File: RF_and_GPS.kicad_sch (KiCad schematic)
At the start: 34 parts, among them J12 U.FL-R-SMT-1, J2 U.FL-R-SMT-1, J29 Conn_02x05_Odd_Even, J7 U.FL-R-SMT-1, Q21 IRF7404, Q38 IRLML2803, Q9 IRLML2803, SW2 KMR231NG LFS, U11 MAX706RESA+, U13 EP2W+, U14 S1216V8, U23 RFM98PW, U9 ATSAMD21E18A-A

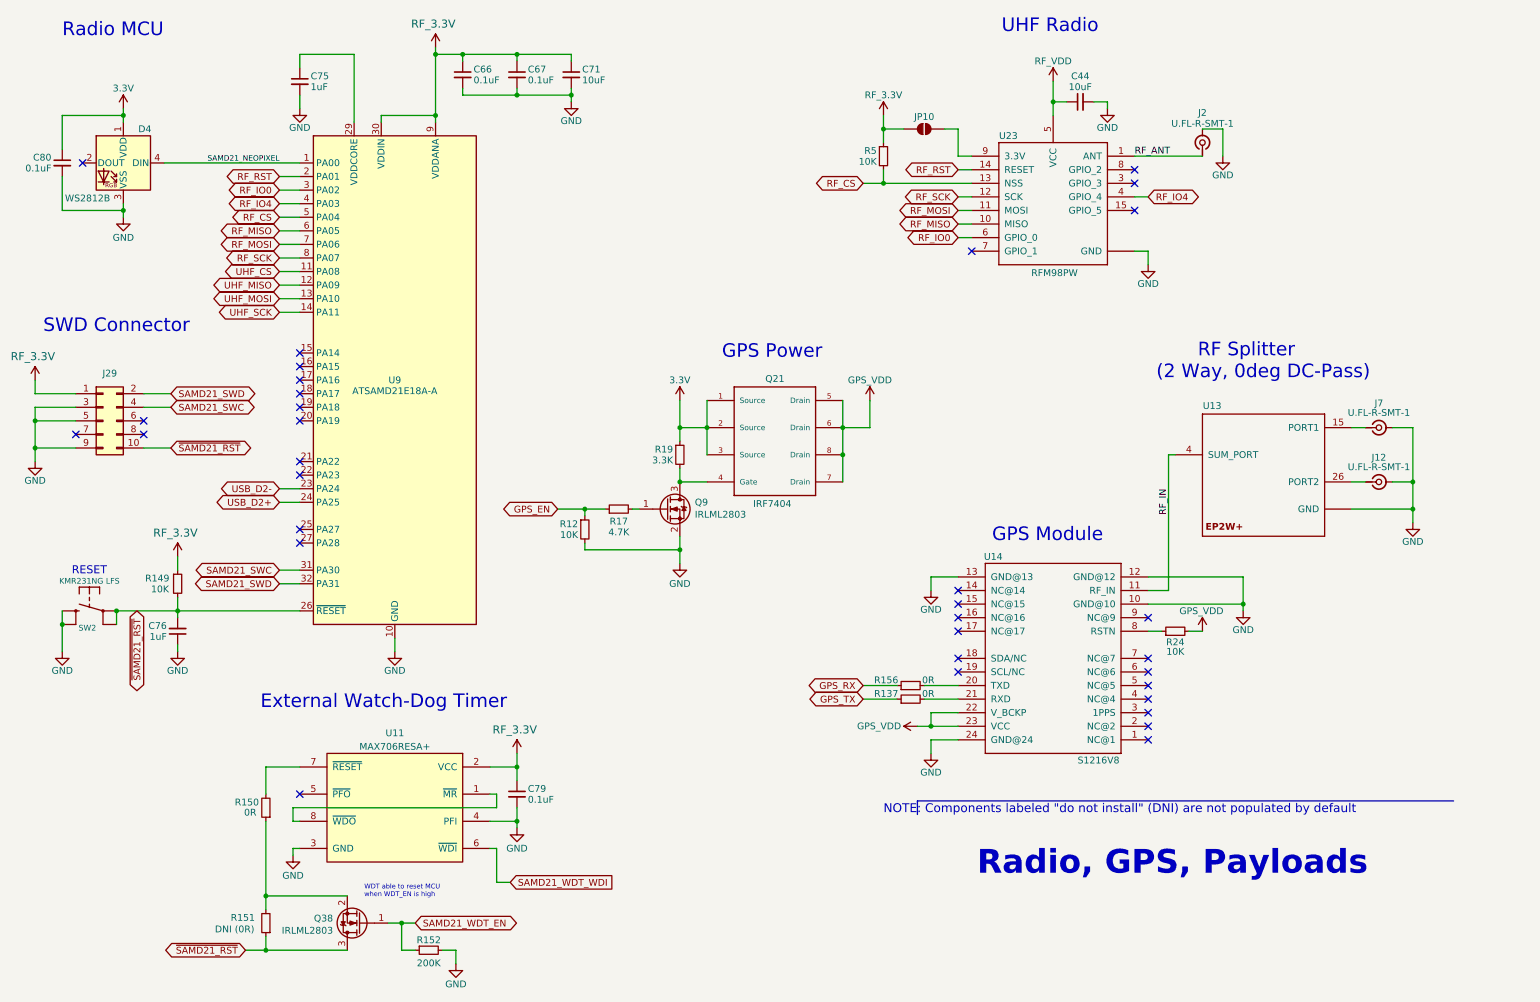
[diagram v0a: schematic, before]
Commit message: Complete layout
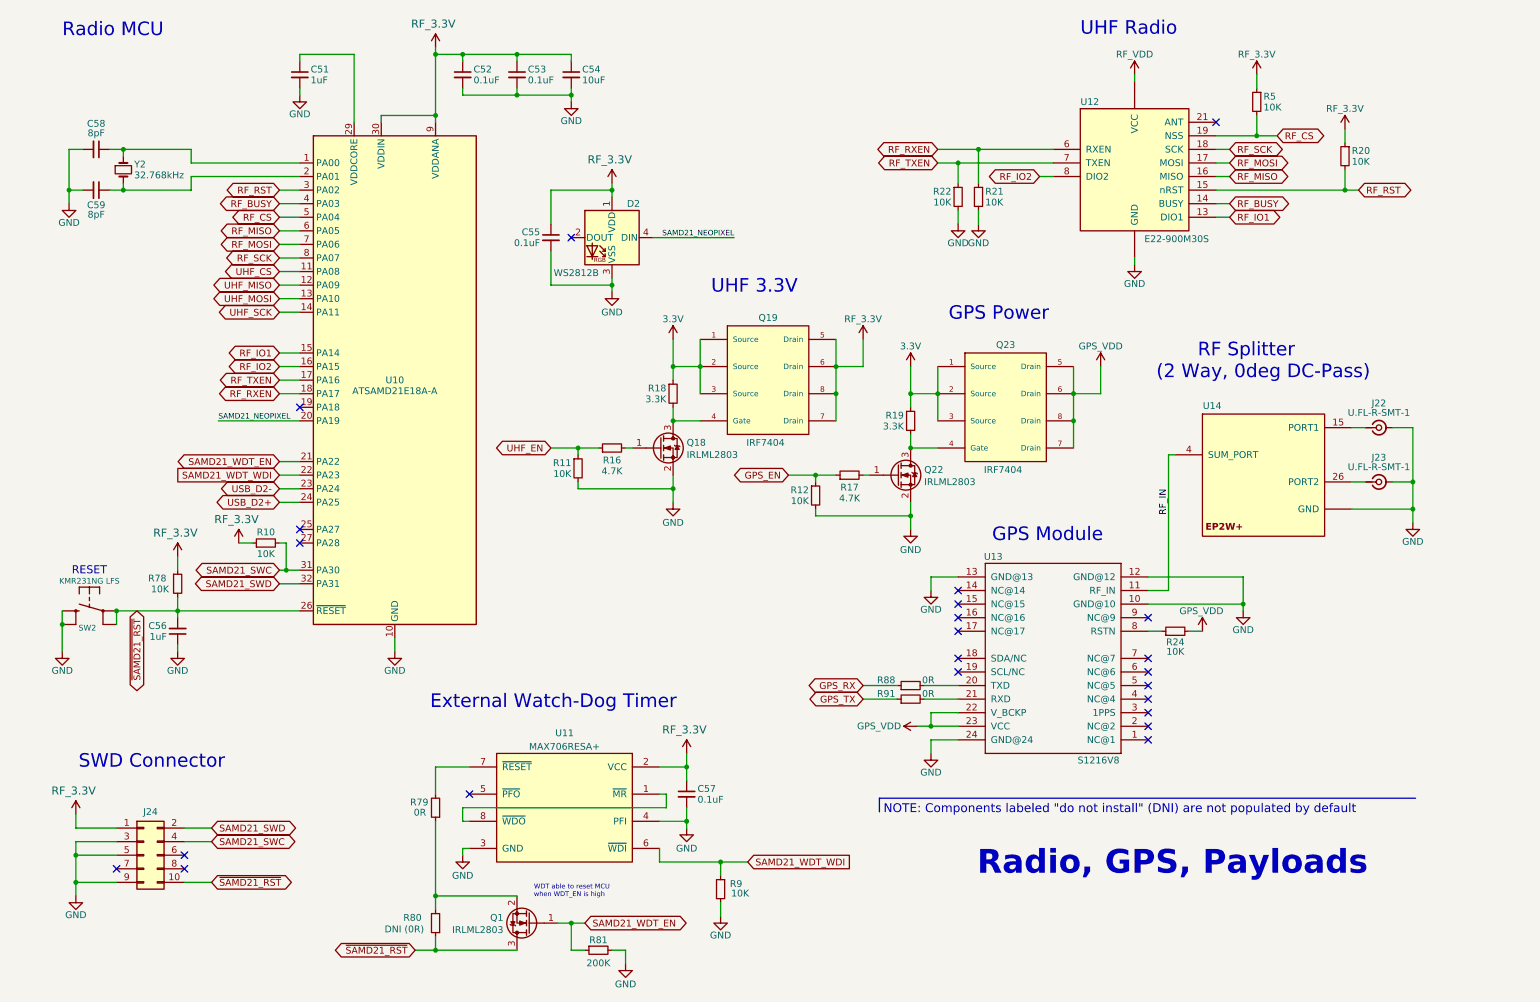
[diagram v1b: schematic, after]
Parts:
- removed C44: 10uF, symbol Device:C_Small
- removed J2: U.FL-R-SMT-1, symbol Connector:Conn_Coaxial_Small
- removed JP10: SolderJumper_2_Open, symbol Jumper:SolderJumper_2_Open
- added C58, C59: 8pF, Capacitor_SMD:C_0603_1608Metric, symbol Device:C_Small
- added Q18: IRLML2803, Package_TO_SOT_SMD:SOT-23, symbol Mainboard:IRLML2803
- added Q19: IRF7404, Package_SO:SOIC-8_3.9x4.9mm_P1.27mm, symbol Mainboard:IRF7404
- added R10, R11, R20, R21, R22, R9: 10K, Resistor_SMD:R_0603_1608Metric, symbol Device:R_Small
- added R16: 4.7K, Resistor_SMD:R_0603_1608Metric, symbol Device:R_Small
- added R18: 3.3K, Resistor_SMD:R_0603_1608Metric, symbol Device:R_Small
- added Y2: 32.768kHz, Crystal:Crystal_SMD_3215-2Pin_3.2x1.5mm, symbol Device:Crystal_Small
- C51: renamed from C75; footprint (none) -> Capacitor_SMD:C_0603_1608Metric
- C52: renamed from C66; footprint (none) -> Capacitor_SMD:C_0603_1608Metric
- C53: renamed from C67; footprint (none) -> Capacitor_SMD:C_0603_1608Metric
- C54: renamed from C71; footprint (none) -> Capacitor_SMD:C_0603_1608Metric
- C55: renamed from C80; symbol mainboard:C_Small -> Device:C_Small
- C56: renamed from C76; symbol mainboard:C_Small -> Device:C_Small
- J22: renamed from J7; footprint (none) -> Connector_Coaxial:U.FL_Hirose_U.FL-R-SMT-1_Vertical
- J23: renamed from J12; footprint (none) -> Connector_Coaxial:U.FL_Hirose_U.FL-R-SMT-1_Vertical
- J24: renamed from J29; footprint (none) -> Connector_PinHeader_1.27mm:PinHeader_2x05_P1.27mm_Vertical_SMD
- Q1: renamed from Q38; symbol Transistor_FET:IRLML2060 -> Mainboard:IRLML2803
- Q22: renamed from Q9; symbol Transistor_FET:IRLML2060 -> Mainboard:IRLML2803
- Q23: renamed from Q21; footprint mainboard:NDS8434 -> Package_SO:SOIC-8_3.9x4.9mm_P1.27mm; symbol mainboard:NDS8434 -> Mainboard:IRF7404
- R88: renamed from R156; footprint (none) -> Resistor_SMD:R_0603_1608Metric
- R91: renamed from R137; footprint (none) -> Resistor_SMD:R_0603_1608Metric
- SW2: footprint mainboard:BTN_KMR2_4.6X2.8 -> Button_Switch_SMD:SW_Push_1P1T_NO_CK_KMR2; symbol mainboard:SWITCH_SMT4.6X2.8 -> Mainboard:KMR231
- U11: symbol mainboard:MAX708RESA+ -> Mainboard:MAX706RESA+
- U12: renamed from U23; value RFM98PW -> E22-900M30S; footprint mainboard:RFM95PW -> mainboard:XCVR_E22-900M30S; symbol mainboard:RFM98PW -> Mainboard:E22-900M30S
- U13: renamed from U14; symbol mainboard:S1216V8 -> Mainboard:S1216V8
- U14: renamed from U13; footprint mainboard:QFN32-5X5MM -> mainboard:EP2W+; symbol mainboard:EP2W+ -> Mainboard:EP2W+
- renumbered C79 to C57, D4 to D2, R149 to R78, R150 to R79, R151 to R80, R152 to R81, U9 to U10
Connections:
- net RF_ANT is gone; now on net GND: U12.1 (GND)
- net 3.3V: now also Q19.1 (Source), Q19.2 (Source), Q19.3 (Source), R18.1; no longer C55.1, D2.1 (VDD)
- net GND: now also SW2.2 (S1), U12.11 (GND), U12.12 (GND), U12.20 (GND), U12.22 (GND), U12.3 (GND), U12.4 (GND), U12.5 (GND), C58.2, C59.2, Q18.2 (S), R11.2, R21.2, R22.2, R9.2; no longer SW2.B (S), SW2.B' (S1), U12.16 (GND), U12.17 (GND)
- net RF_3.3V: now also C55.1, D2.1 (VDD), Q19.5 (Drain), Q19.6 (Drain), Q19.7 (Drain), Q19.8 (Drain), R10.1, R20.1
- net RF_CS: now also U12.19 (NSS); no longer U12.13 (NSS)
- net RF_MISO: now also U12.16 (MISO); no longer U12.10 (MISO)
- net RF_MOSI: now also U12.17 (MOSI); no longer U12.11 (MOSI)
- net RF_RST: now also U10.3 (PA02), U12.15 (nRST), R20.2; no longer U10.2 (PA01), U12.14 (RESET)
- net RF_SCK: now also U12.18 (SCK); no longer U12.12 (SCK)
- net RF_VDD: now also U12.10 (VCC), U12.9 (VCC); no longer U12.5 (VCC)
- net SAMD21_NEOPIXEL: now also U10.20 (PA19); no longer U10.1 (PA00)
- net SAMD21_SWC: now also R10.2
- net SAMD21_WDT_EN: now also U10.21 (PA22)
- net SAMD21_WDT_WDI: now also U10.22 (PA23), R9.1
- net ~{SAMD21_RST}: now also SW2.1 (P1); no longer SW2.A (P), SW2.A' (P1)
- net RF_TXEN: now reaches U12.7 (TXEN)
- net RF_TXEN: now also U10.17 (PA16), R22.1
- net RF_IO2: now reaches U12.8 (DIO2)
- net RF_IO2: now also U10.16 (PA15)
- net RF_IO1: now reaches U10.15 (PA14)
- net RF_IO1: now also U12.13 (DIO1)
- net RF_RXEN: now reaches U10.18 (PA17)
- net RF_RXEN: now also U12.6 (RXEN), R21.1
- removed net RF_IO0: U10.3 (PA02), U12.6 (GPIO_0)
- net RF_IO4 renamed RF_BUSY
- net RF_BUSY: now also U12.14 (BUSY); no longer U12.4 (GPIO_4)
- new net: C58.1, U10.1 (PA00), Y2.1
- new net: Q18.3 (D), Q19.4 (Gate), R18.2
- new net: C59.1, U10.2 (PA01), Y2.2
- new net: Q18.1 (G), R16.2
- new net UHF_EN: R11.1, R16.1
- no-connect marks 33 -> 23
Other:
- note added: "UHF 3.3V"
- moved on the sheet: C51, C55, C57, D2, J24, Q1, Q22, R12, R17, R19, R5, R79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
